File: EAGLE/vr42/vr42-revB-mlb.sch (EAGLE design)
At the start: 82 parts, among them U1 2N7002, U2 2N7002, U3 74AHCT1G125GW, U33 USB3300-EZK, X1 12MHz, X2 32.768MHz, X3 24MHz

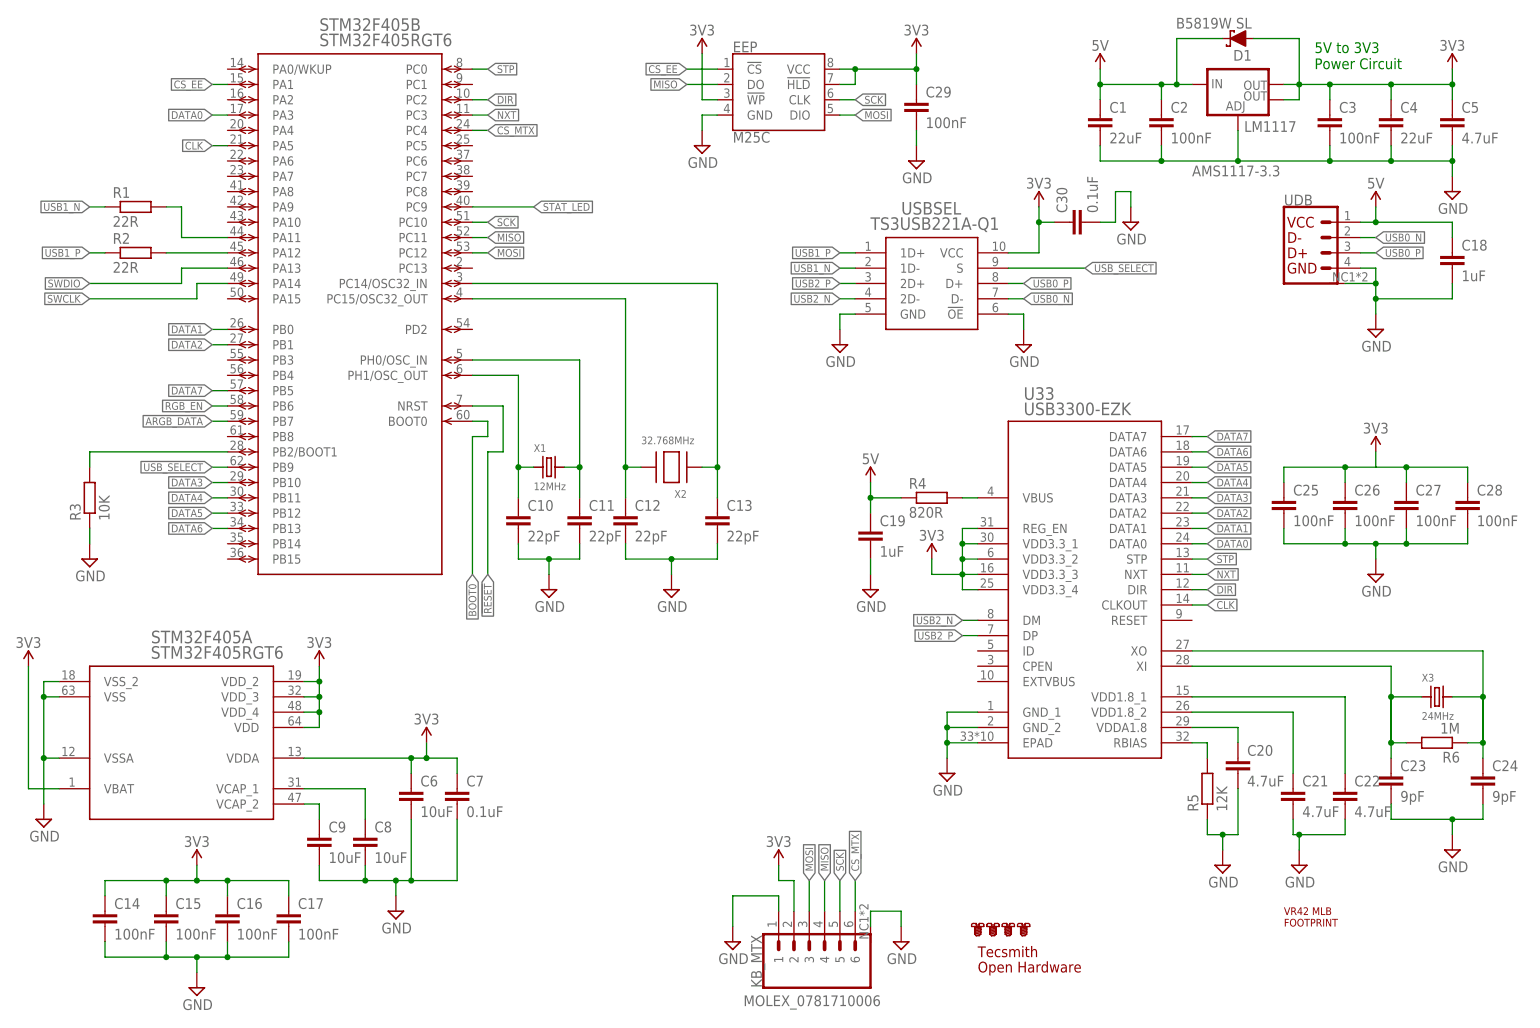
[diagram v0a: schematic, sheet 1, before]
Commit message: .
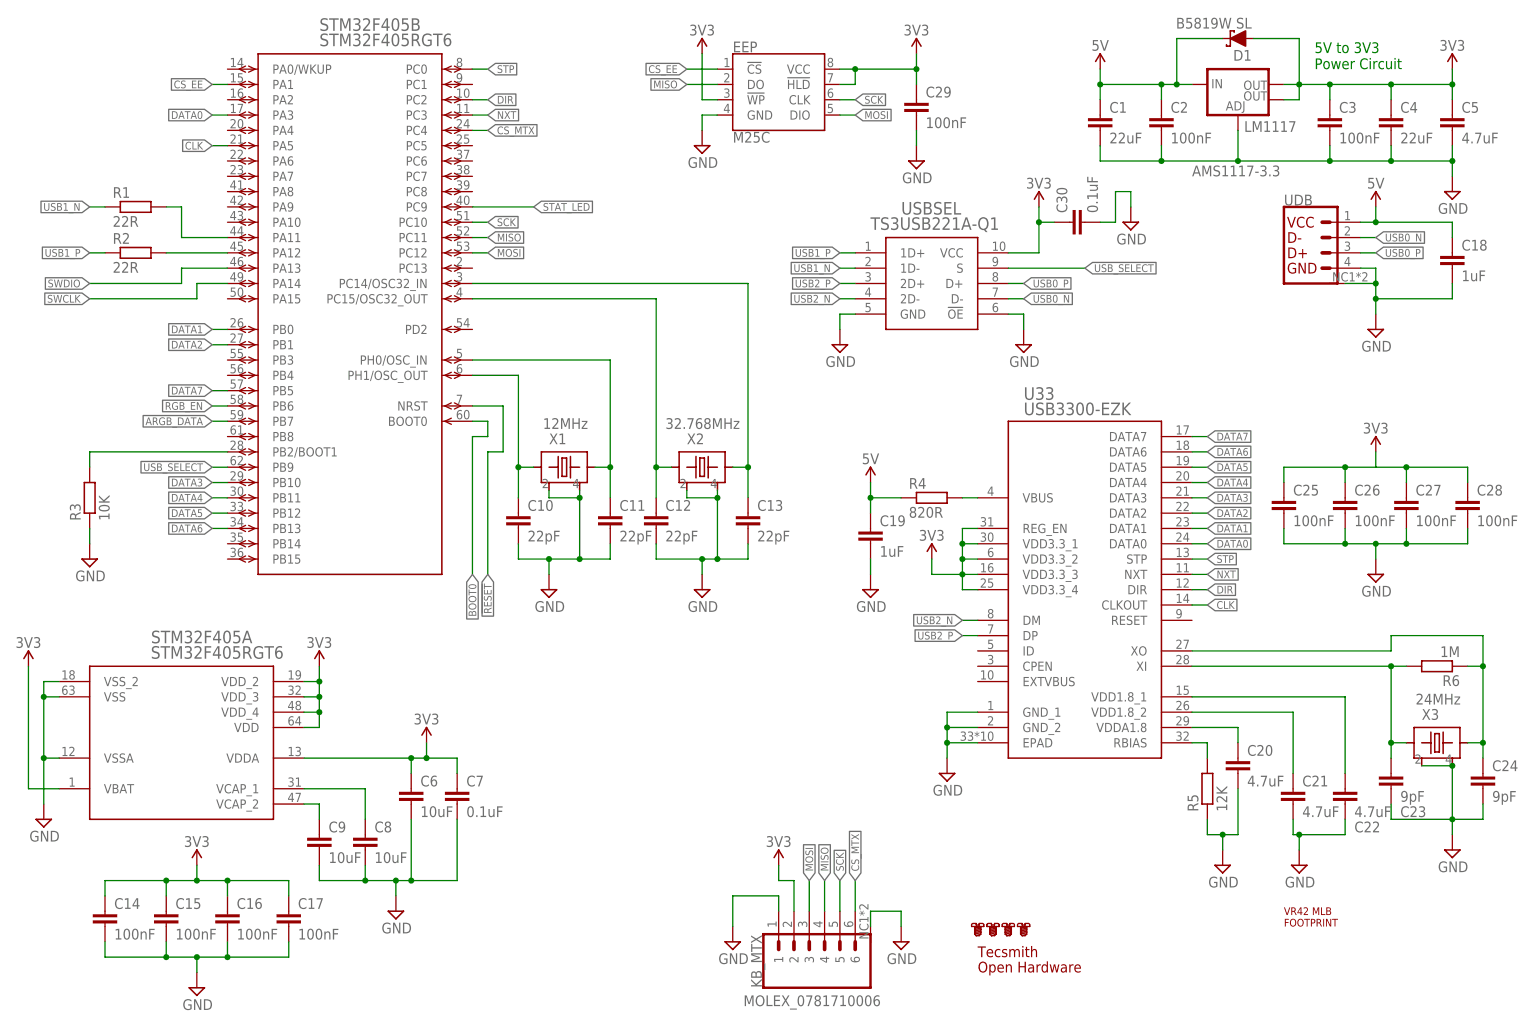
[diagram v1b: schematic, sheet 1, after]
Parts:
- X1, X3: device microbuilder:CRYSTAL2.5X2.0 -> __temp_to_delete:CRYSTAL2.5X2.0
- X2: device adafruit2:XTAL-3.2X1.5 -> __temp_to_delete:CRYSTAL2.5X2.0
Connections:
- net GND: now also X1.2, X1.4, X2.2, X2.4, X3.2, X3.4
- net N$10: now also X3.3; no longer X3.2
- net OSC32_IN: now also X2.3; no longer X2.P$1
- net OSC32_OUT: now also X2.1; no longer X2.P$2
- net OSC_IN: now also X1.3; no longer X1.2
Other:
- moved on the sheet: C11, C12, C13, R6
